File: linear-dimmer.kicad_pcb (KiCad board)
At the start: 2 copper layers, 49.3 x 30.4 mm, 32 parts, among them CON1 AVR-ISP-6, IC1 ATTINY85-S, P1 POWER, P2 OUTPUT, Q1 Q_NMOS_GDS, SW1 ENCODER, U1 LM78L05ACZ, U2 MCP6401

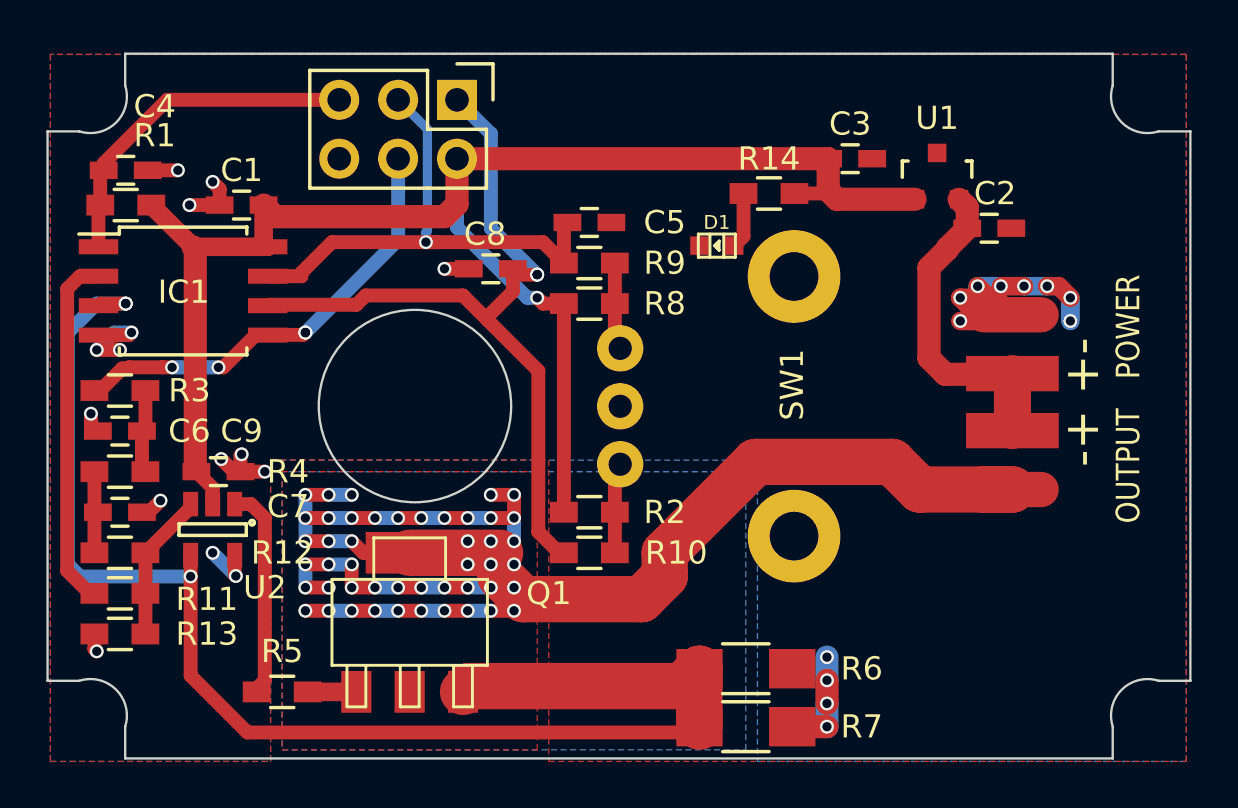
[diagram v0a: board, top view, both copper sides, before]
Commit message: Shuffle stuff around, generate gerbers
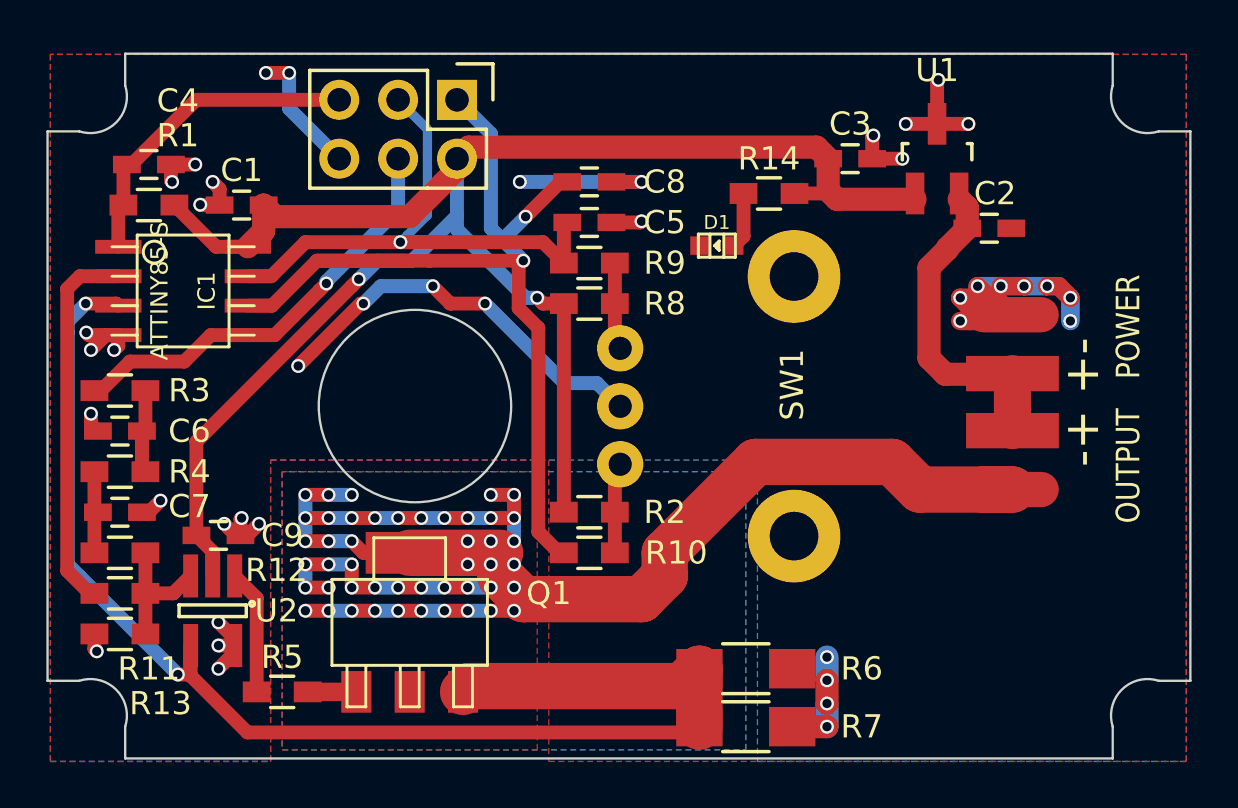
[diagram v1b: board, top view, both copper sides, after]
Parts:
- IC1: footprint Housings_SOIC:SOIJ-8_5.3x5.3mm_Pitch1.27mm -> w_smd_dil:so-8
- U1: footprint Housings_SOT-23_SOT-143_TSOT-6:SOT-23 -> Housings_SOT-23_SOT-143_TSOT-6:SOT-23_Handsoldering
- moved C8 5.67 mm to (133.2, 75.5), turned to 0 degrees
- moved U2 3.50 mm to (117.0, 94.0)
- moved C9 2.75 mm to (117.2, 90.8)
- moved C4 1.03 mm to (114.2, 74.8)
- moved R1 1.00 mm to (114.2, 76.5)
- moved U1 0.75 mm to (148.2, 74.5)
- turned IC1 to 270 degrees
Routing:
- net GND: track 37.3 -> 74.2 mm, vias 27 -> 42
- net +5V: track 70.3 -> 78.4 mm, vias 1 -> 2
- net Net-(C8-Pad1): track 34.4 -> 42.1 mm
- net Net-(IC1-Pad3): track 61.5 -> 57.8 mm, vias 3 -> 2
- net Net-(R5-Pad1): track 9.19 -> 5.54 mm
- net Net-(C5-Pad1): track 22.8 -> 25.2 mm
- net Net-(C4-Pad1): track 15.0 -> 14.0 mm
- net Net-(IC1-Pad2): track 15.3 -> 16.2 mm
- net Net-(R11-Pad1): track 6.61 -> 5.76 mm
- net Net-(CON1-Pad4): track 19.3 -> 18.6 mm, vias 4 -> 1
